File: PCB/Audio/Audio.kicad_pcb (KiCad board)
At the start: 2 copper layers, 70 x 70 mm, 32 parts, among them J3 TC2030-USB-NL-DS, J4 TF_PUSH, J5 USB-C-Socket-H, U1 L, U2 R, U6 ESP32-S3-MINI-1, U7 MD8942

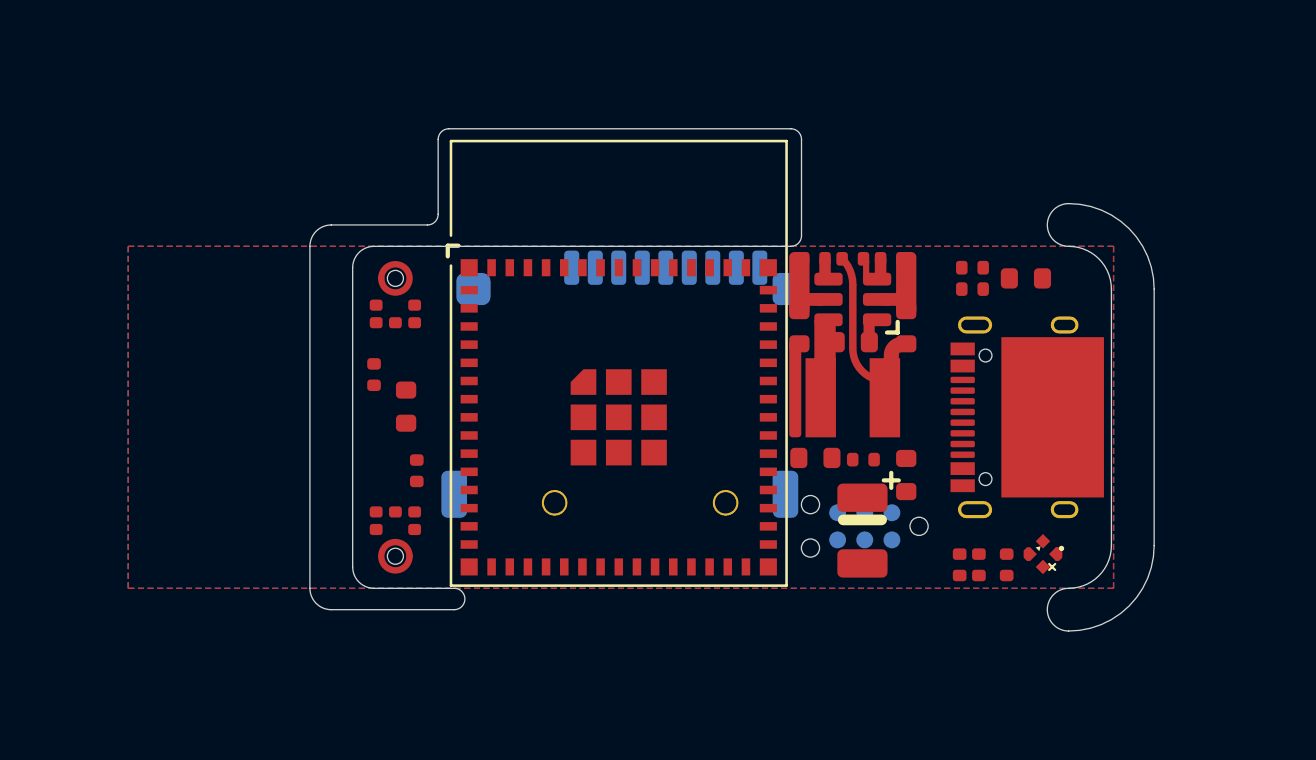
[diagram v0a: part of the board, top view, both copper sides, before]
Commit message: Closer
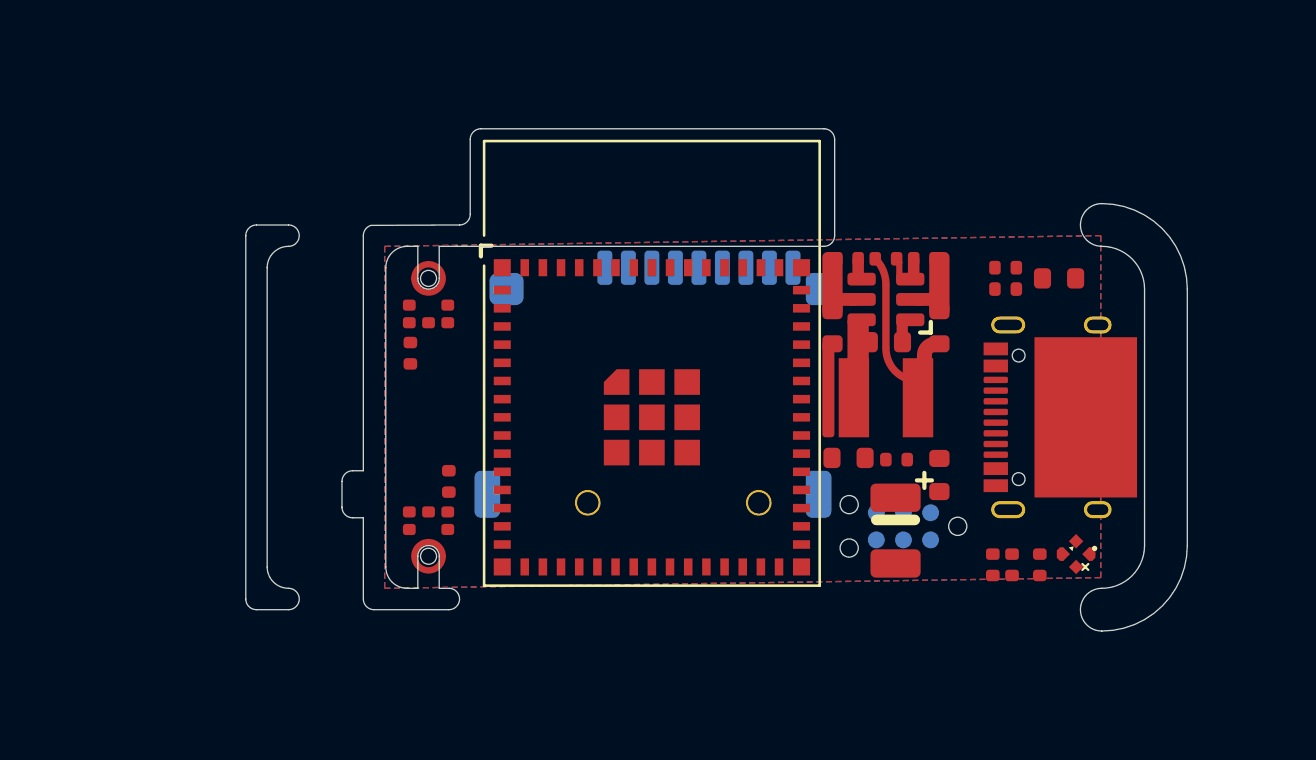
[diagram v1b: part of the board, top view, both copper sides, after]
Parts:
- removed C6: 10uF 35V, RevK:C_0603
- V2: moved to B.Cu
- moved C8 1.97 mm to (88.7, 97.0)
- moved J3 1.81 mm to (111.8, 105.1)
- moved C13 1.58 mm to (90.5, 103.0)
- moved C1 1.55 mm to (111.4, 105.3)
- moved C2 1.55 mm to (111.4, 102.0)
- moved C4 1.55 mm to (118.2, 106.9)
- moved R15 1.55 mm to (109.2, 92.6)
- moved C10 1.55 mm to (108.5, 95.8)
- moved C11 1.55 mm to (113.5, 95.8)
- moved C12 1.55 mm to (111.0, 96.5)
- moved C3 1.55 mm to (109.2, 101.9)
- moved C5 1.55 mm to (113.5, 102.7)
- moved C7 1.55 mm to (119.0, 93.5)
- moved C9 1.55 mm to (116.5, 94.0)
- moved D1 1.55 mm to (119.8, 106.4)
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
